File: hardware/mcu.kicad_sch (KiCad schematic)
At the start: 23 parts, among them J101 Conn_ARM_JTAG_SWD_10, SW101 SW_Push, U101 EFR32FG28A122F1024GM48-A, Y101 LF_Crystal, Y102 ECS-390-CDX-1932

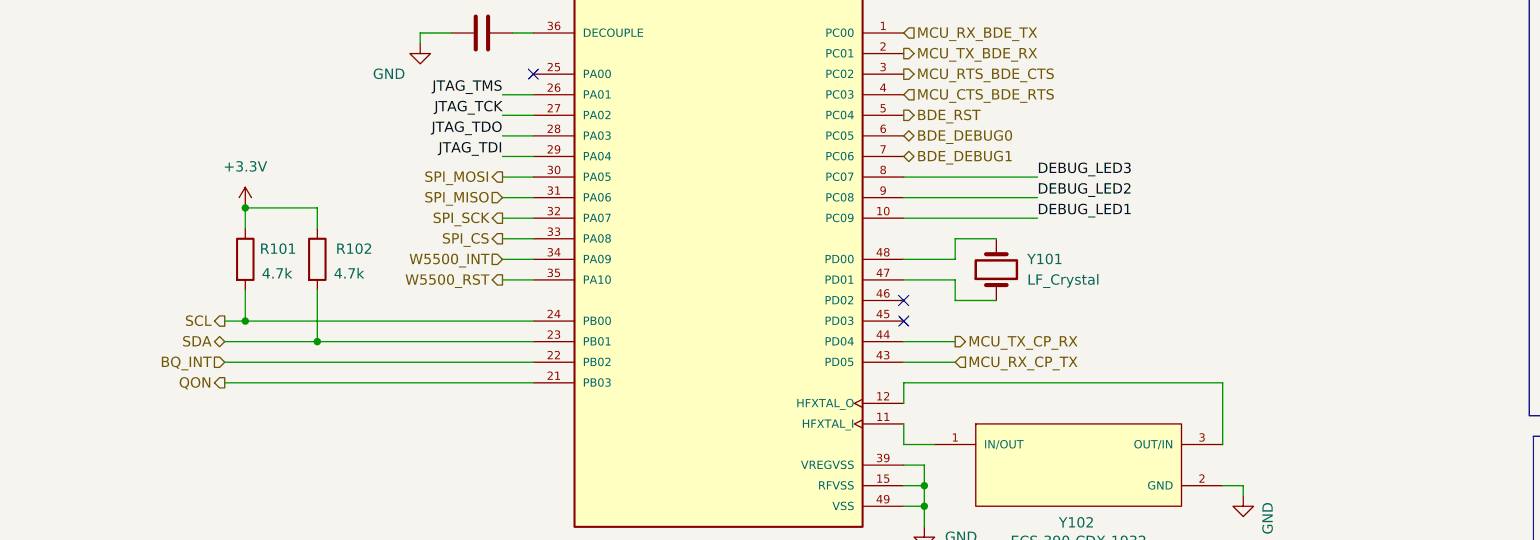
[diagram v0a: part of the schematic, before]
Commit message: MCU pin update
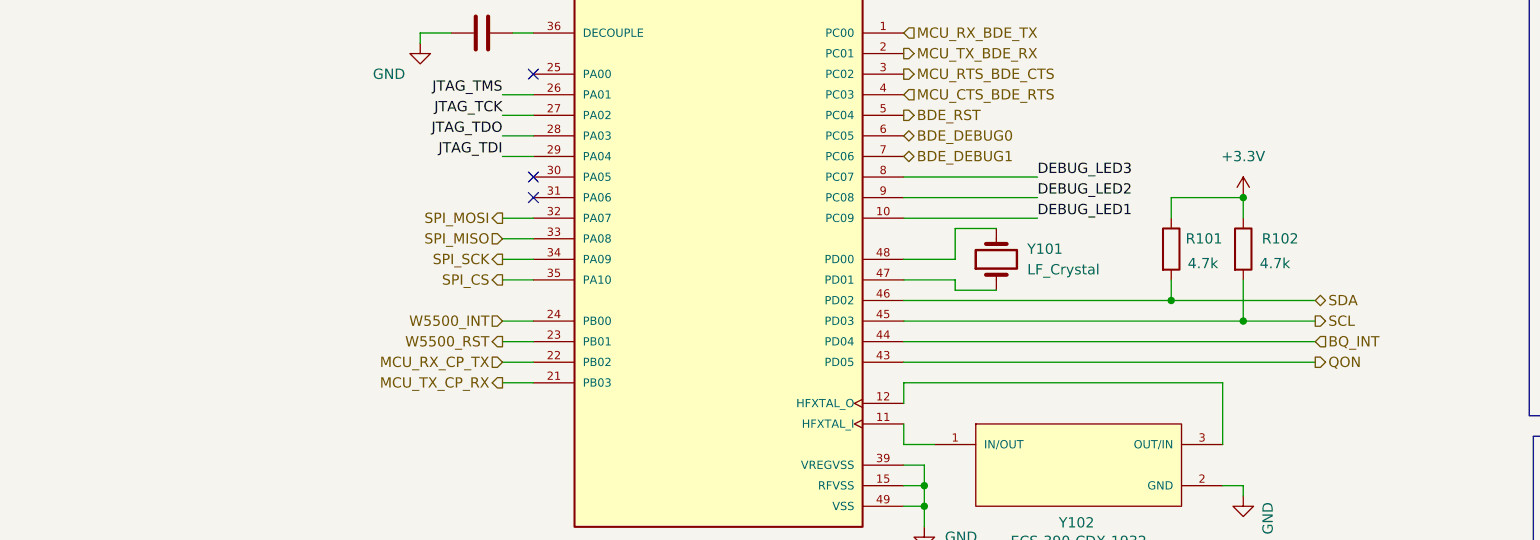
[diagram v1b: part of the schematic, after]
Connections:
- net BQ_INT: now also U101.44 (PD04); no longer U101.22 (PB02)
- net MCU_RX_CP_TX: now also U101.22 (PB02); no longer U101.43 (PD05)
- net MCU_TX_CP_RX: now also U101.21 (PB03); no longer U101.44 (PD04)
- net QON: now also U101.43 (PD05); no longer U101.21 (PB03)
- net SCL: now also R102.2, U101.45 (PD03); no longer R101.2, U101.24 (PB00)
- net SDA: now also R101.2, U101.46 (PD02); no longer R102.2, U101.23 (PB01)
- net SPI_CS: now also U101.35 (PA10); no longer U101.33 (PA08)
- net SPI_MISO: now also U101.33 (PA08); no longer U101.31 (PA06)
- net SPI_MOSI: now also U101.32 (PA07); no longer U101.30 (PA05)
- net SPI_SCK: now also U101.34 (PA09); no longer U101.32 (PA07)
- net W5500_INT: now also U101.24 (PB00); no longer U101.34 (PA09)
- net W5500_RST: now also U101.23 (PB01); no longer U101.35 (PA10)
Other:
- moved on the sheet: R101, R102, Y101
